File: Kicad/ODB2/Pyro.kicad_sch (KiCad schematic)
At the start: 32 parts, among them U11 TLV172IDCK, U12 74LVC2G08DP_125, U13 74AHC1G04, U14 TLV172IDCK

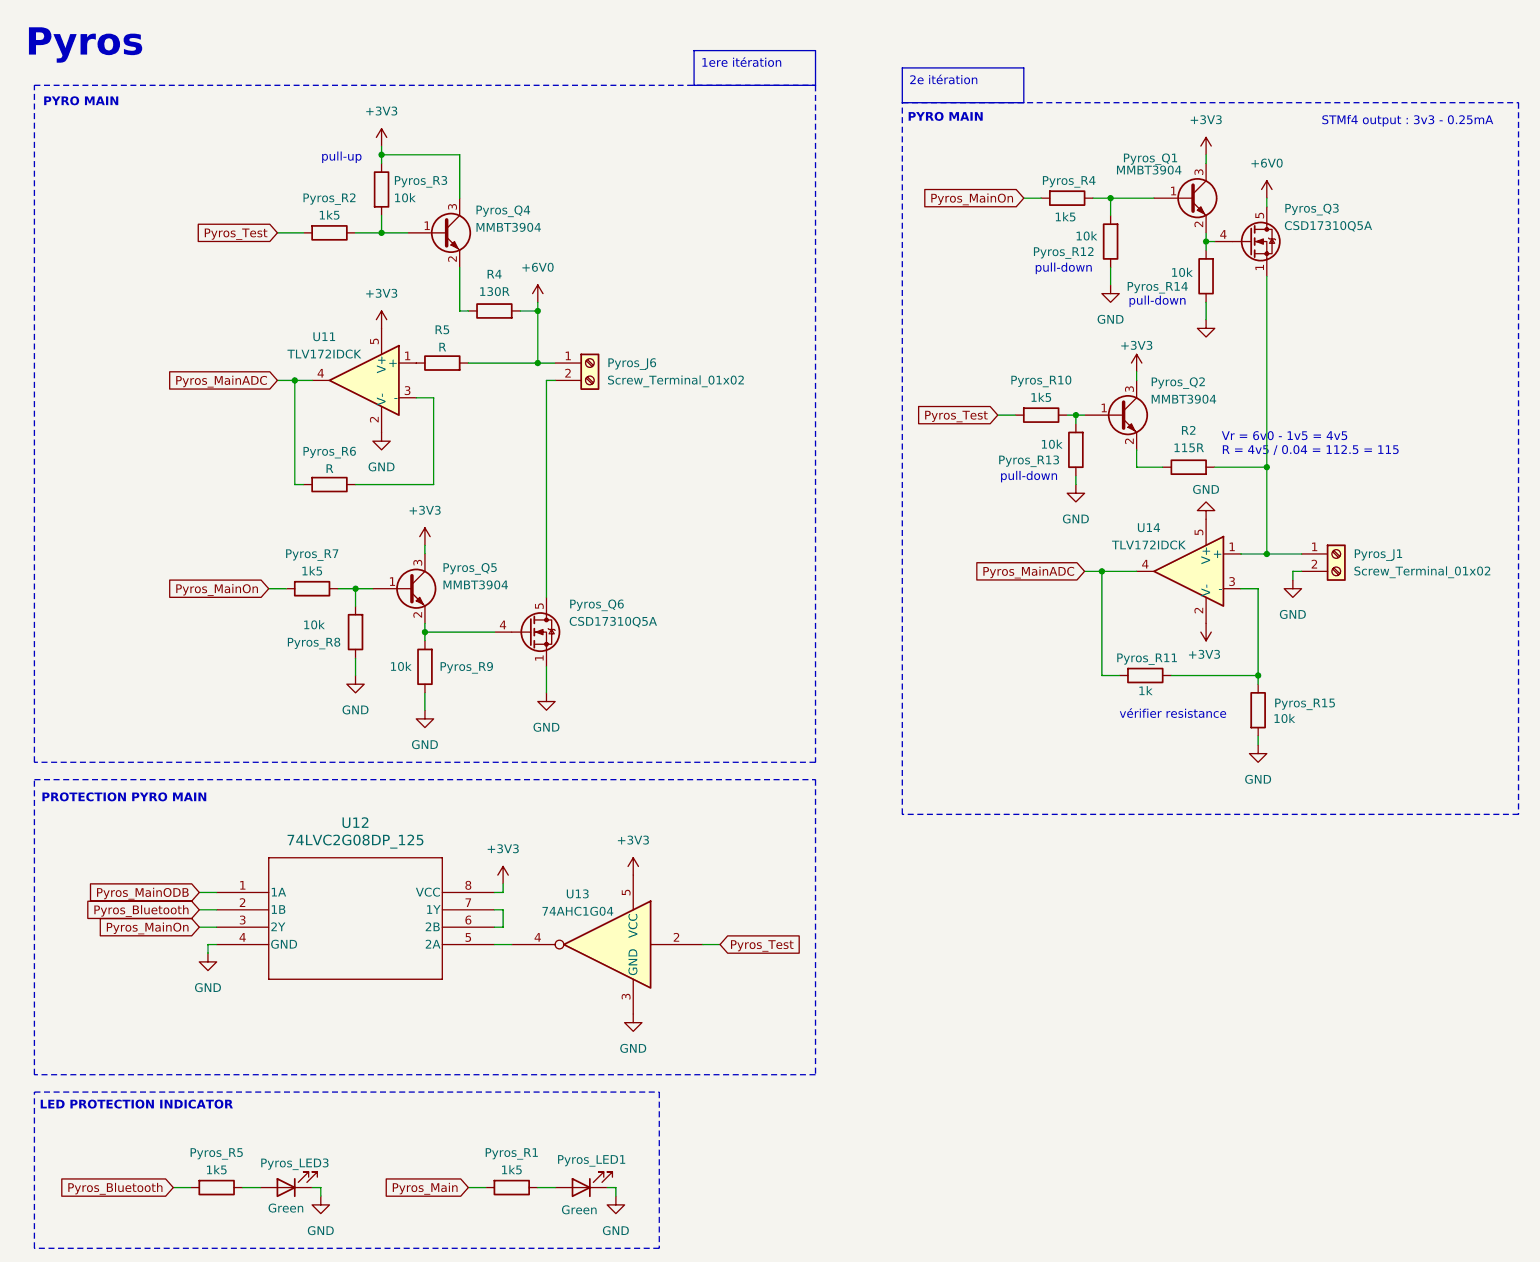
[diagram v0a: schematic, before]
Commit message: pyros
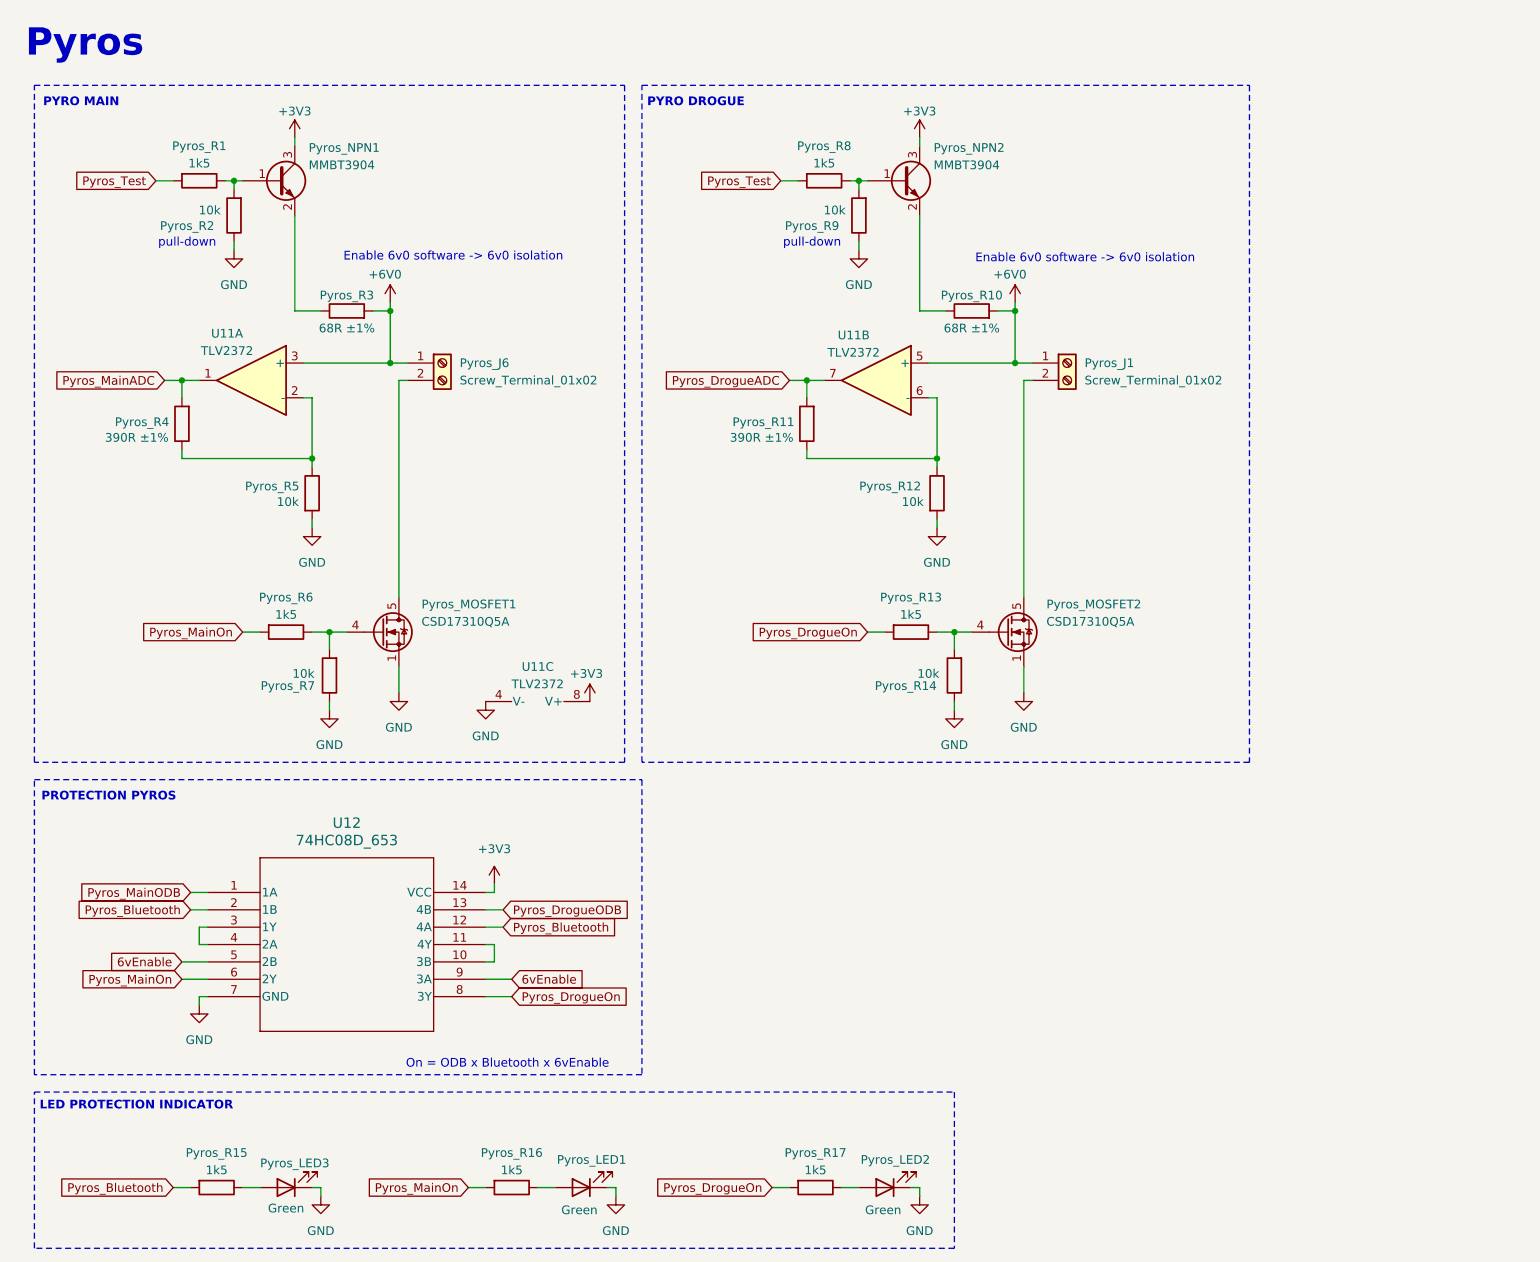
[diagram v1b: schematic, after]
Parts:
- removed Pyros_Q1, Pyros_Q2, Pyros_Q4, Pyros_Q5: MMBT3904, Package_TO_SOT_SMD:SOT-23, symbol Transistor_BJT:MMBT3904
- removed Pyros_Q3: CSD17310Q5A, Package_TO_SOT_SMD:TDSON-8-1, symbol Transistor_FET:CSD17310Q5A
- removed Pyros_R15, Pyros_R3: 10k, symbol Device:R
- removed Pyros_R6, R5: R, symbol Device:R
- removed R2: 115R, symbol Device:R
- removed U11, U14: TLV172IDCK, Package_TO_SOT_SMD:SOT-353_SC-70-5, symbol Amplifier_Operational:TLV172IDCK
- removed U12: 74LVC2G08DP_125, TSSOP8_SOT505-2_NEX, symbol ODB_Lib:74LVC2G08DP_125
- removed U13: 74AHC1G04, symbol 74xGxx:74AHC1G04
- added Pyros_LED2: Green, symbol Device:LED
- added Pyros_MOSFET2: CSD17310Q5A, Package_TO_SOT_SMD:TDSON-8-1, symbol Transistor_FET:CSD17310Q5A
- added Pyros_NPN1, Pyros_NPN2: MMBT3904, Package_TO_SOT_SMD:SOT-23, symbol Transistor_BJT:MMBT3904
- added Pyros_R1, Pyros_R17, Pyros_R8: 1k5, symbol Device:R
- added Pyros_R5: 10k, symbol Device:R
- added U11: TLV2372, symbol Amplifier_Operational:TLV2372
- added U12: 74HC08D_653, SO14_SOT108-1_NEX, symbol ODB_Lib:74HC08D_653
- Pyros_R10: value 1k5 -> 68R ±1%
- Pyros_R11: value 1k -> 390R ±1%
- Pyros_R13: value 10k -> 1k5
- Pyros_R2: value 1k5 -> 10k
- Pyros_R3: renamed from R4; value 130R -> 68R ±1%
- Pyros_R4: value 1k5 -> 390R ±1%
- renumbered Pyros_Q6 to Pyros_MOSFET1, Pyros_R5 to Pyros_R15, Pyros_R1 to Pyros_R16, Pyros_R7 to Pyros_R6, Pyros_R8 to Pyros_R7
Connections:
- net Pyros_Main is gone; now on net Pyros_MainOn: Pyros_R16.2
- net +3V3: now also Pyros_NPN1.3 (C), Pyros_NPN2.3 (C), U11.8 (V+), U12.14 (VCC)
- net +6V0: now also Pyros_J1.1 (Pin_1), Pyros_R10.2, U11.3 (+), U11.5 (+)
- net GND: now also Pyros_R12.2, Pyros_R2.1, Pyros_LED2.1 (K), Pyros_MOSFET2.1 (S), Pyros_MOSFET2.2 (S), Pyros_MOSFET2.3 (S), Pyros_R5.2, U11.4 (V-), U12.7 (GND); no longer Pyros_J1.2 (Pin_2), Pyros_R12.1, Pyros_R13.1
- net Pyros_Bluetooth: now also U12.12 (4A), U12.2 (1B)
- net Pyros_MainADC: now also Pyros_R4.2, U11.1; no longer Pyros_R11.2
- net Pyros_MainODB: now also U12.1 (1A)
- net Pyros_MainOn: now also U12.6 (2Y); no longer Pyros_R4.2
- net Pyros_Test: now also Pyros_R1.2, Pyros_R8.2; no longer Pyros_R10.2, Pyros_R2.2
- net at Pyros_R4.1: now also Pyros_R5.1, U11.2 (-); no longer Pyros_R12.2
- net at Pyros_R10.1: now also Pyros_NPN2.2 (E); no longer Pyros_R13.2
- net at Pyros_R6.1, Pyros_R7.2: now also Pyros_MOSFET1.4 (G)
- net at Pyros_R9.2: now also Pyros_NPN2.1 (B), Pyros_R8.1; no longer Pyros_MOSFET1.4 (G)
- net at Pyros_R14.2: now also Pyros_R13.1, Pyros_MOSFET2.4 (G)
- net at Pyros_R11.1: now also Pyros_R12.1, U11.6 (-)
- net at Pyros_R3.1: now also Pyros_NPN1.2 (E)
- new net: Pyros_J1.2 (Pin_2), Pyros_MOSFET2.5 (D)
- new net: U12.10 (3B), U12.11 (4Y)
- new net: U12.3 (1Y), U12.4 (2A)
- new net: Pyros_NPN1.1 (B), Pyros_R1.1, Pyros_R2.2
- new net: Pyros_LED2.2 (A), Pyros_R17.1
- new net 6vEnable: U12.5 (2B), U12.9 (3A)
- new net Pyros_DrogueADC: Pyros_R11.2, U11.7
- new net Pyros_DrogueODB: U12.13 (4B)
- new net Pyros_DrogueOn: Pyros_R13.2, Pyros_R17.2, U12.8 (3Y)
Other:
- note added: "Enable 6v0 software -> 6v0 isolation"
- note added: "On = ODB x Bluetooth x 6vEnable"
- note added: "PROTECTION PYROS"
- note added: "PYRO DROGUE"
- note removed: "PROTECTION PYRO MAIN"
- note removed: "STMf4 output : 3v3 - 0.25mA"
- note removed: "Vr = 6v0 - 1v5 = 4v5 R = 4v5 / 0.04 = 112.5 = 115"
- note removed: "pull-up"
- note removed: "vérifier resistance"
- moved on the sheet: Pyros_J6, Pyros_MOSFET1, Pyros_R3, Pyros_R6, Pyros_R7

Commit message: fix and gate
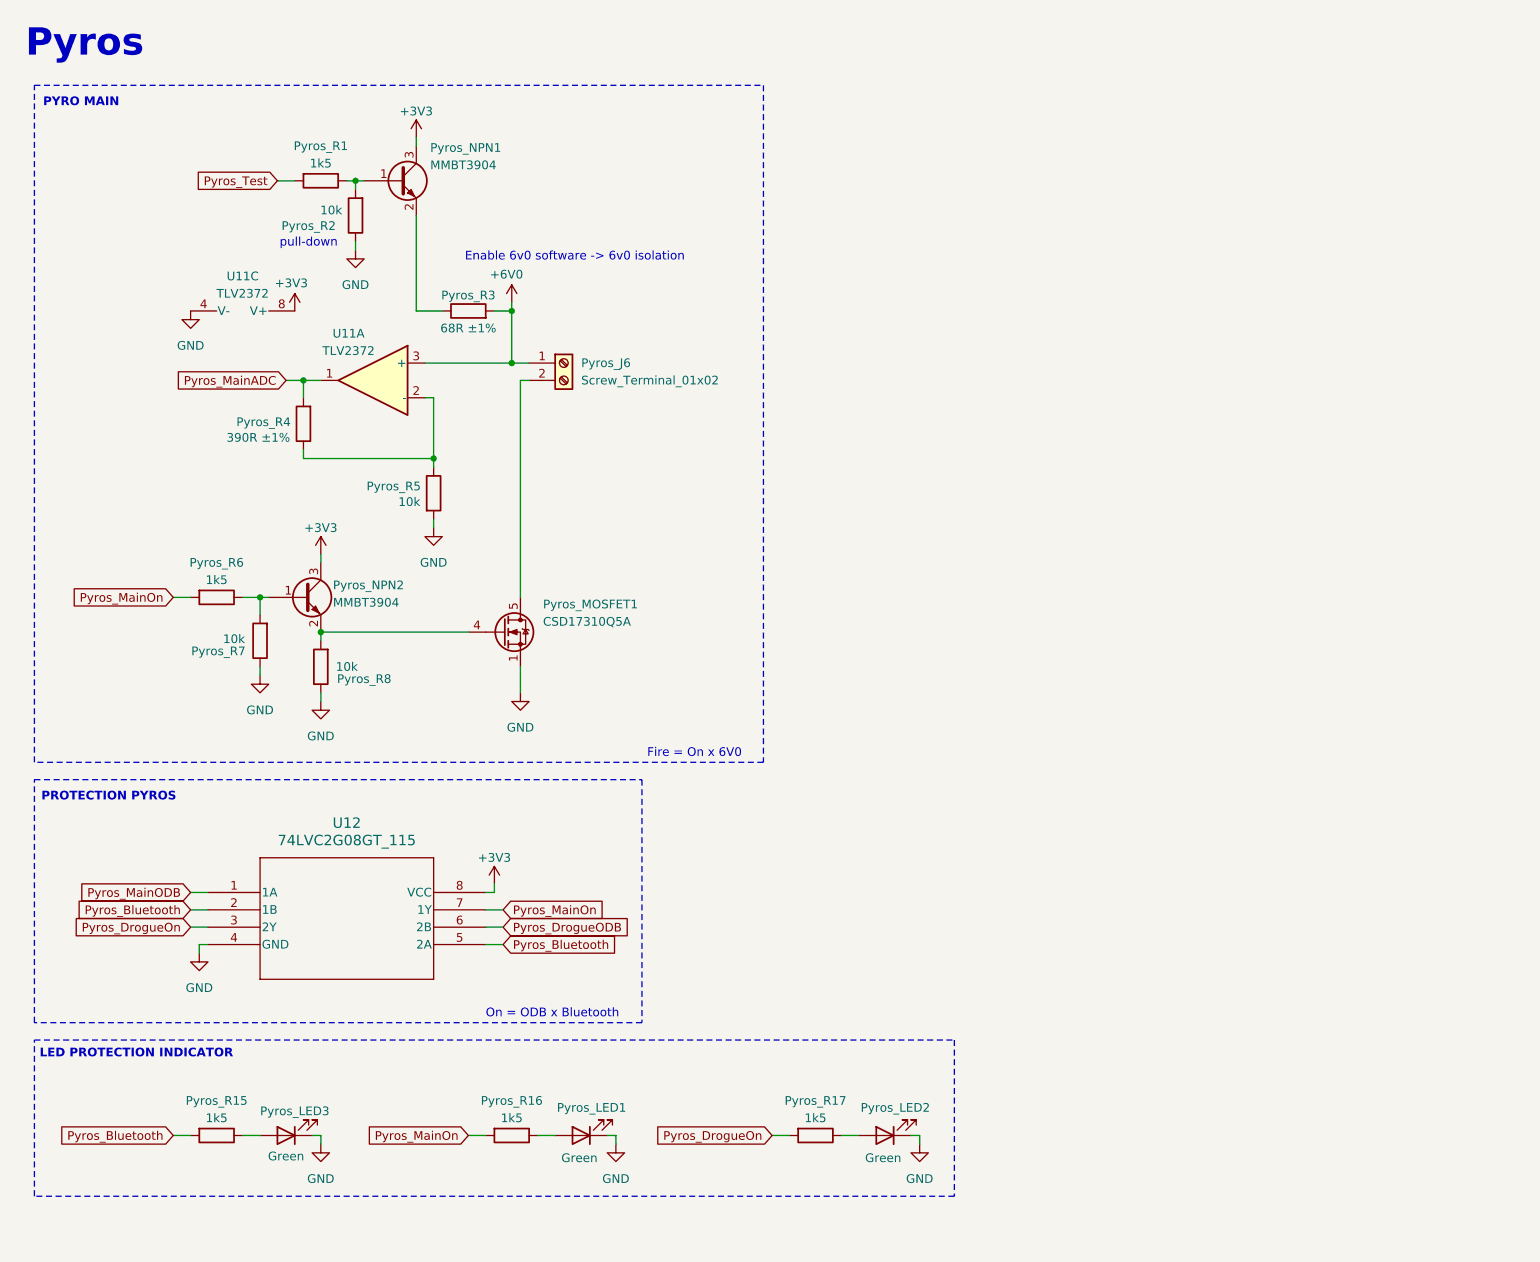
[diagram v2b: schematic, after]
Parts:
- removed Pyros_J1: Screw_Terminal_01x02, symbol Connector:Screw_Terminal_01x02
- removed Pyros_MOSFET2: CSD17310Q5A, Package_TO_SOT_SMD:TDSON-8-1, symbol Transistor_FET:CSD17310Q5A
- removed Pyros_R10: 68R ±1%, symbol Device:R
- removed Pyros_R11: 390R ±1%, symbol Device:R
- removed Pyros_R12, Pyros_R14, Pyros_R9: 10k, symbol Device:R
- removed Pyros_R13: 1k5, symbol Device:R
- removed unit 2 of U11
- removed U12: 74HC08D_653, SO14_SOT108-1_NEX, symbol ODB_Lib:74HC08D_653
- added U12: 74LVC2G08GT_115, Library:XSON8_SOT833-1_NEX, symbol ODB_Lib:74LVC2G08GT_115
- Pyros_R8: value 1k5 -> 10k
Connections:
- net +3V3: now also U12.8 (VCC)
- net GND: now also Pyros_R8.1, U12.4 (GND)
- net Pyros_Bluetooth: now also U12.2 (1B), U12.5 (2A)
- net Pyros_DrogueODB: now also U12.6 (2B)
- net Pyros_DrogueOn: now also U12.3 (2Y)
- net Pyros_MainODB: now also U12.1 (1A)
- net Pyros_MainOn: now also U12.7 (1Y)
- net Pyros_Test: no longer Pyros_R8.2
- net at Pyros_R6.1, Pyros_R7.2: now also Pyros_NPN2.1 (B); no longer Pyros_MOSFET1.4 (G)
- net at Pyros_NPN2.2 (E): now also Pyros_MOSFET1.4 (G), Pyros_R8.2
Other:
- note added: "Fire = On x 6V0"
- note added: "On = ODB x Bluetooth"
- note removed: "On = ODB x Bluetooth x 6vEnable"
- note removed: "PYRO DROGUE"
- moved on the sheet: Pyros_J6, Pyros_LED1, Pyros_LED2, Pyros_LED3, Pyros_MOSFET1, Pyros_NPN1, Pyros_R1, Pyros_R15, Pyros_R16, Pyros_R17, Pyros_R2, Pyros_R3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
